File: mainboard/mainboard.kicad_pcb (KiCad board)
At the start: 2 copper layers, 100 x 110 mm, 428 parts, among them J1 USB_B_Micro, J2 Conn_01x02_MountingPin, J3 Conn_01x19_MountingPin, J4 Conn_01x19_MountingPin, Q1 DMG2301L, Q2 MMBT3904, Q3 MMBT3904, SW1 SW_Push, SW2 SW_Push, U1 tps63070, U2 tps63070, U3 tps63070, U4 BME680, U5 LIS3MDL, U6 BH1750FVI, U7 CP2102N-A01-GQFN24, U8 ESP32-WROOM-32, U9 ADXL343

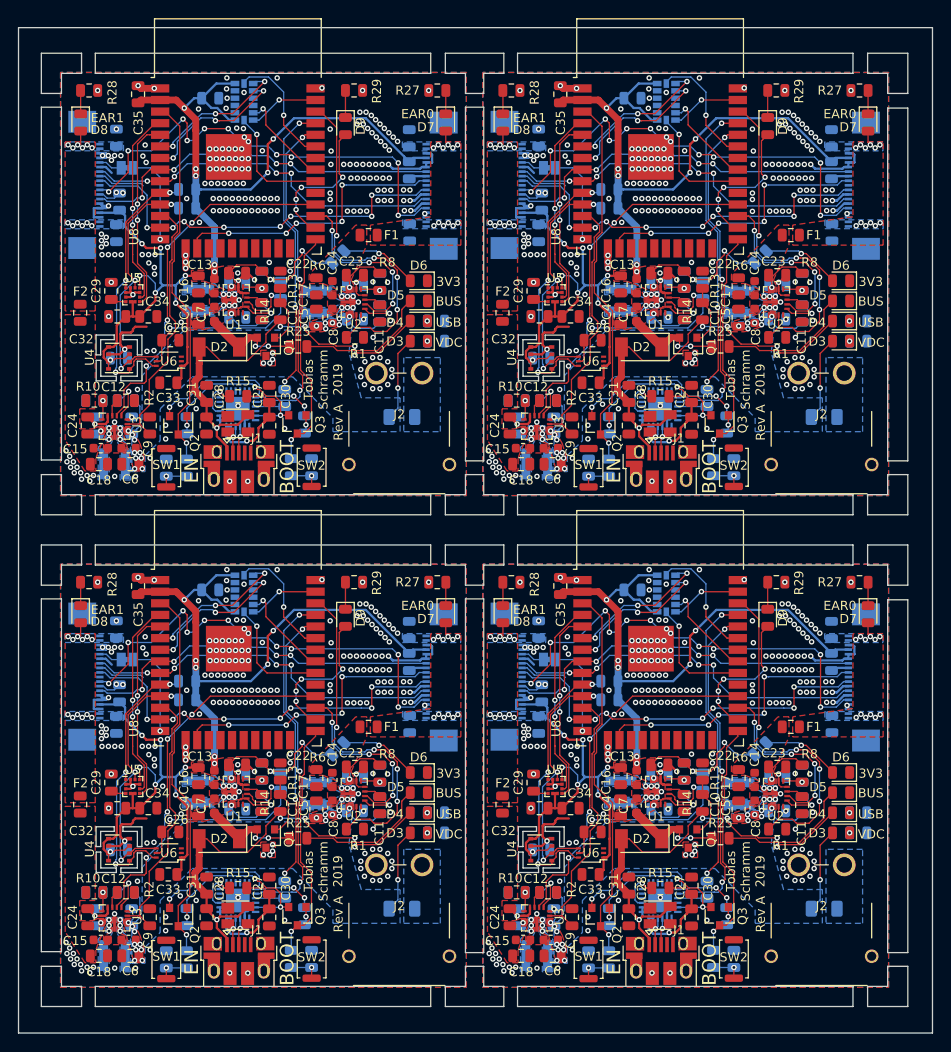
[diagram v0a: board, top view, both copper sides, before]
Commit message: Add allignment holes
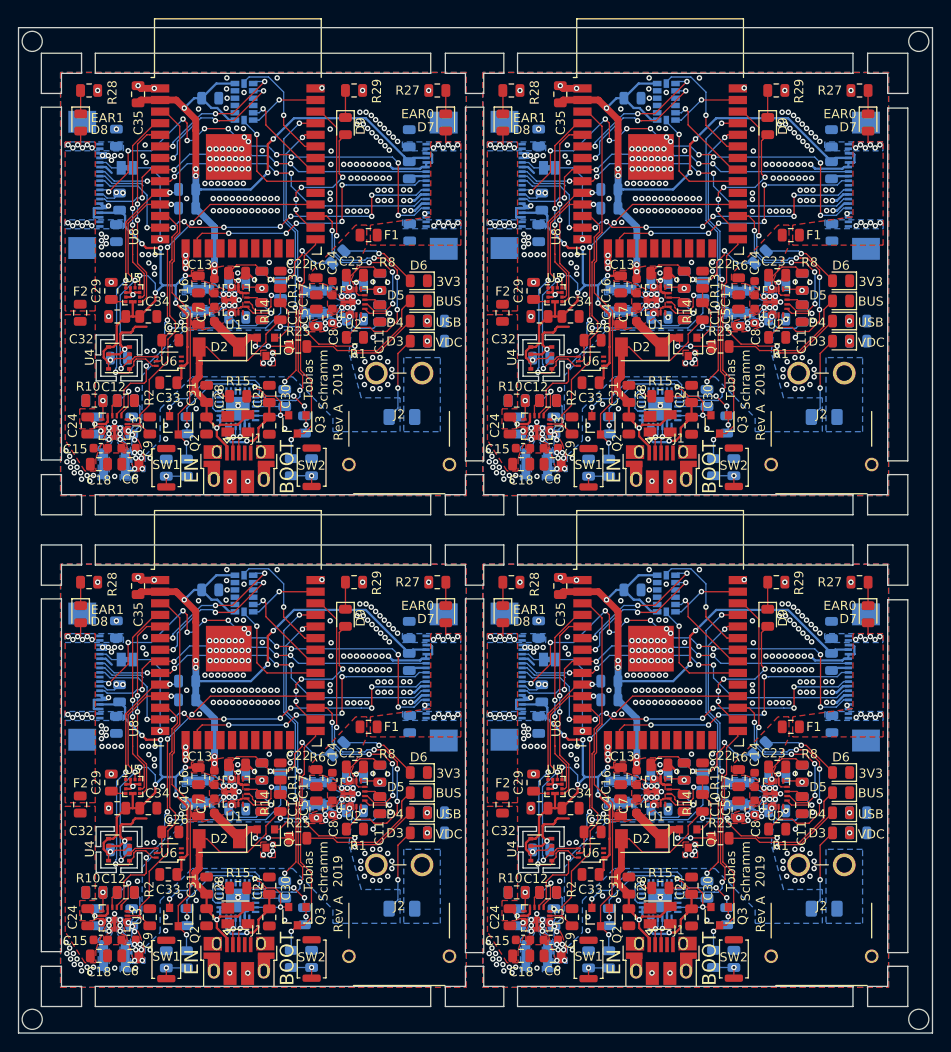
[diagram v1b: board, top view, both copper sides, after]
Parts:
- added REF**: Allignment_Hole, mainboard:Allignment_Hole, F.Cu at (118.5, 128.5)
- added REF**: Allignment_Hole, mainboard:Allignment_Hole, F.Cu at (21.5, 128.5)
- added REF**: Allignment_Hole, mainboard:Allignment_Hole, F.Cu at (21.5, 21.5)
- added REF**: Allignment_Hole, mainboard:Allignment_Hole, F.Cu at (118.5, 21.5)
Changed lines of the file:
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@@
     (tracks 4952)
     (zones 0)
-    (modules 428)
+    (modules 432)
     (nets 95)
   )
@@
   )
   (setup
-    (last_trace_width 0.25)
+    (last_trace_width 0.127)
     (user_trace_width 0.127)
     (user_trace_width 0.25)
@@
     (add_net VUSB)
   )
+  (module mainboard:Allignment_Hole (layer F.Cu)
+    (at 118.5 128.5)
+    (fp_text reference REF** (at 0 3.25) (layer F.SilkS) hide
+      (effects (font (size 1 1) (thickness 0.15)))
+    )
+    (fp_text value Allignment_Hole (at 0 -3.25) (layer F.Fab)
+      (effects (font (size 1 1) (thickness 0.15)))
+    )
+    (fp_circle (center 0 0) (end 2.2 0) (layer Cmts.User) (width 0.15))
+    (fp_circle (center 0 0) (end 2.45 0) (layer F.CrtYd) (width 0.05))
+    (pad "" np_thru_hole circle (at 0 0) (size 2.2 2.2) (drill 2.2) (layers *.Cu *.Paste *.Mask))
+  )
+  (module mainboard:Allignment_Hole (layer F.Cu)
+    (at 21.5 128.5)
+    (fp_text reference REF** (at 0 3.25) (layer F.SilkS) hide
+      (effects (font (size 1 1) (thickness 0.15)))
+    )
+    (fp_text value Allignment_Hole (at 0 -3.25) (layer F.Fab)
+      (effects (font (size 1 1) (thickness 0.15)))
+    )
+    (fp_circle (center 0 0) (end 2.2 0) (layer Cmts.User) (width 0.15))
+    (fp_circle (center 0 0) (end 2.45 0) (layer F.CrtYd) (width 0.05))
+    (pad "" np_thru_hole circle (at 0 0) (size 2.2 2.2) (drill 2.2) (layers *.Cu *.Paste *.Mask))
+  )
+  (module mainboard:Allignment_Hole (layer F.Cu)
+    (at 21.5 21.5)
+    (fp_text reference REF** (at 0 3.25) (layer F.SilkS) hide
+      (effects (font (size 1 1) (thickness 0.15)))
+    )
+    (fp_text value Allignment_Hole (at 0 -3.25) (layer F.Fab)
+      (effects (font (size 1 1) (thickness 0.15)))
+    )
+    (fp_circle (center 0 0) (end 2.2 0) (layer Cmts.User) (width 0.15))
+    (fp_circle (center 0 0) (end 2.45 0) (layer F.CrtYd) (width 0.05))
+    (pad "" np_thru_hole circle (at 0 0) (size 2.2 2.2) (drill 2.2) (layers *.Cu *.Paste *.Mask))
+  )
+  (module mainboard:Allignment_Hole (layer F.Cu)
+    (at 118.5 21.5)
+    (fp_text reference REF** (at 0 3.25) (layer F.SilkS) hide
+      (effects (font (size 1 1) (thickness 0.15)))
+    )
+    (fp_text value Allignment_Hole (at 0 -3.25) (layer F.Fab)
+      (effects (font (size 1 1) (thickness 0.15)))
+    )
+    (fp_circle (center 0 0) (end 2.2 0) (layer Cmts.User) (width 0.15))
+    (fp_circle (center 0 0) (end 2.45 0) (layer F.CrtYd) (width 0.05))
+    (pad "" np_thru_hole circle (at 0 0) (size 2.2 2.2) (drill 2.2) (layers *.Cu *.Paste *.Mask))
+  )
   (module Resistor_SMD:R_0805_2012Metric (layer B.Cu)
